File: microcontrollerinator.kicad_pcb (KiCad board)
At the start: 2 copper layers, 21 x 51 mm, 47 parts, among them J1 USB_C_Receptacle_USB2.0_14P, J2 Conn_01x20, J3 Conn_01x20, J4 Conn_01x03, J5 Conn_01x03, Q1 AO3401A, SW1 SW_Push, U1 RP2040, U2 MCP1700x-330xxTT, U3 W25Q128JVS, U4 BQ21040DBV, Y1 12MHz

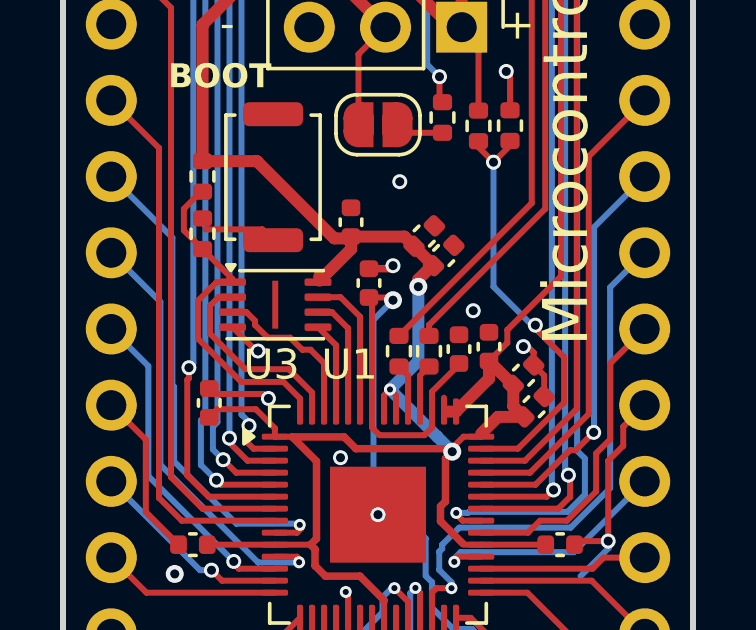
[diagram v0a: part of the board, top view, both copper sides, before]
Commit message: fixed pcb
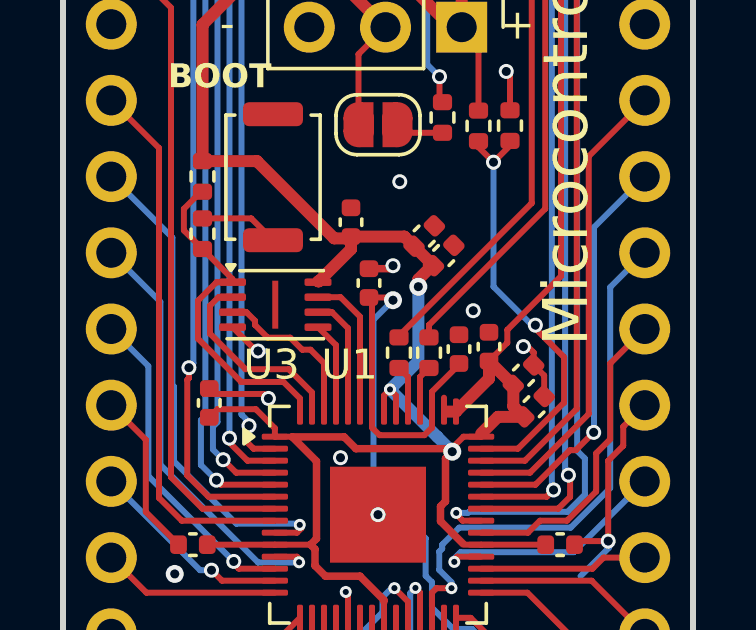
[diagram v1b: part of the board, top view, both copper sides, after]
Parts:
- R3, R4: value 27K -> 27
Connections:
- C13 pad 1: /VBAT -> Net-(U2-VI)
- U2 pad 3: /VBAT -> Net-(U2-VI)
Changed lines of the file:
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@@
 	(net 59 "/QSPI_SD3")
 	(net 60 "/QSPI_SD1")
+	(net 61 "Net-(U2-VI)")
 	(footprint "Crystal:Crystal_SMD_3225-4Pin_3.2x2.5mm"
 		(layer "F.Cu")
@@
 			(layers "F.Cu" "F.Mask" "F.Paste")
 			(roundrect_rratio 0.25)
-			(net 4 "/VBAT")
+			(net 61 "Net-(U2-VI)")
 			(pinfunction "VI")
 			(pintype "power_in")
@@
 			(layers "F.Cu" "F.Mask" "F.Paste")
 			(roundrect_rratio 0.25)
-			(net 4 "/VBAT")
+			(net 61 "Net-(U2-VI)")
 			(pintype "passive")
 		)
@@
 	(footprint "Resistor_SMD:R_0402_1005Metric"
 		(layer "F.Cu")
-		(at 143.2 105.05 90)
+		(at 143.2 105.1 90)
 		(descr "Resistor SMD 0402 (1005 Metric), square (rectangular) end terminal, IPC-7351 nominal, (Body size source: IPC-SM-782 page 72, https://www.pcb-3d.com/wordpress/wp-content/uploads/ipc-sm-782a_amendment_1_and_2.pdf), generated with kicad-footprint-generator")
 		(tags "resistor")
@@
 			)
 		)
-		(property "Value" "27K"
+		(property "Value" "27"
 			(at 0 1.17 90)
 			(layer "F.Fab")
@@
 	(footprint "Resistor_SMD:R_0402_1005Metric"
 		(layer "F.Cu")
-		(at 142.2 105.05 -90)
+		(at 142.2 105.1 -90)
 		(descr "Resistor SMD 0402 (1005 Metric), square (rectangular) end terminal, IPC-7351 nominal, (Body size source: IPC-SM-782 page 72, https://www.pcb-3d.com/wordpress/wp-content/uploads/ipc-sm-782a_amendment_1_and_2.pdf), generated with kicad-footprint-generator")
 		(tags "resistor")
@@
 			)
 		)
-		(property "Value" "27K"
+		(property "Value" "27"
 			(at 0 1.17 90)
 			(layer "F.Fab")
@@
 	)
 	(segment
+		(start 139.526 102.724)
+		(end 139.5 102.724)
+		(width 0.4)
+		(layer "F.Cu")
+		(net 1)
+	)
+	(segment
 		(start 140.37191 107.907322)
 		(end 138.640452 107.907322)
@@
 	)
 	(segment
-		(start 139.7 102.55)
-		(end 139.55 102.55)
-		(width 0.4)
+		(start 143.975 108.4)
+		(end 143.875 108.3)
+		(width 0.25)
 		(layer "F.Cu")
 		(net 1)
 	)
 	(segment
-		(start 143.975 108.4)
-		(end 143.875 108.3)
-		(width 0.25)
+		(start 140.6 101.65)
+		(end 139.526 102.724)
+		(width 0.4)
 		(layer "F.Cu")
 		(net 1)
@@
 	)
 	(segment
-		(start 139.55 102.55)
-		(end 139.55 102.7)
-		(width 0.4)
-		(layer "F.Cu")
-		(net 1)
-	)
-	(segment
 		(start 141.7 113.9375)
 		(end 141.7 114.9)
@@
 	)
 	(segment
-		(start 140.6 101.65)
-		(end 139.7 102.55)
-		(width 0.4)
-		(layer "F.Cu")
-		(net 1)
-	)
-	(segment
 		(start 139.4 111.65)
 		(end 139.4 112.2)
@@
 	)
 	(segment
-		(start 142.5 105.86)
-		(end 142.2 105.56)
+		(start 142.5 107.0625)
+		(end 142.5 105.91)
 		(width 0.2)
 		(layer "F.Cu")
@@
 	)
 	(segment
-		(start 142.5 106.8625)
-		(end 142.5 105.86)
+		(start 142.5 105.91)
+		(end 142.2 105.61)
 		(width 0.2)
 		(layer "F.Cu")
@@
 	)
 	(segment
-		(start 142.9 105.86)
-		(end 142.9 107.0625)
+		(start 143.15 105.56)
+		(end 143.15 105.75)
+		(width 0.2)
+		(layer "F.Cu")
+		(net 50)
+	)
+	(segment
+		(start 142.9 107.0625)
+		(end 142.9 105.91)
 		(width 0.2)
 		(layer "F.Cu")
@@
 	)
 	(segment
-		(start 143.2 105.56)
-		(end 142.9 105.86)
+		(start 142.9 105.91)
+		(end 143.2 105.61)
 		(width 0.2)
 		(layer "F.Cu")
@@
 	)
 	(segment
-		(start 137.64 100.99)
-		(end 138 101.35)
+		(start 138 101.35)
+		(end 137.275 100.625)
 		(width 0.2)
 		(layer "F.Cu")
@@
 	)
 	(segment
-		(start 135.75 100.99)
-		(end 137.64 100.99)
+		(start 137.275 100.625)
+		(end 135.65 100.625)
 		(width 0.2)
 		(layer "F.Cu")
